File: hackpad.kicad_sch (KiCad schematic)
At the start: 4 parts, among them SW1 SW_Push, SW2 SW_Push, SW3 SW_Push, U1 MOUDLE-SEEEDUINO-XIAO

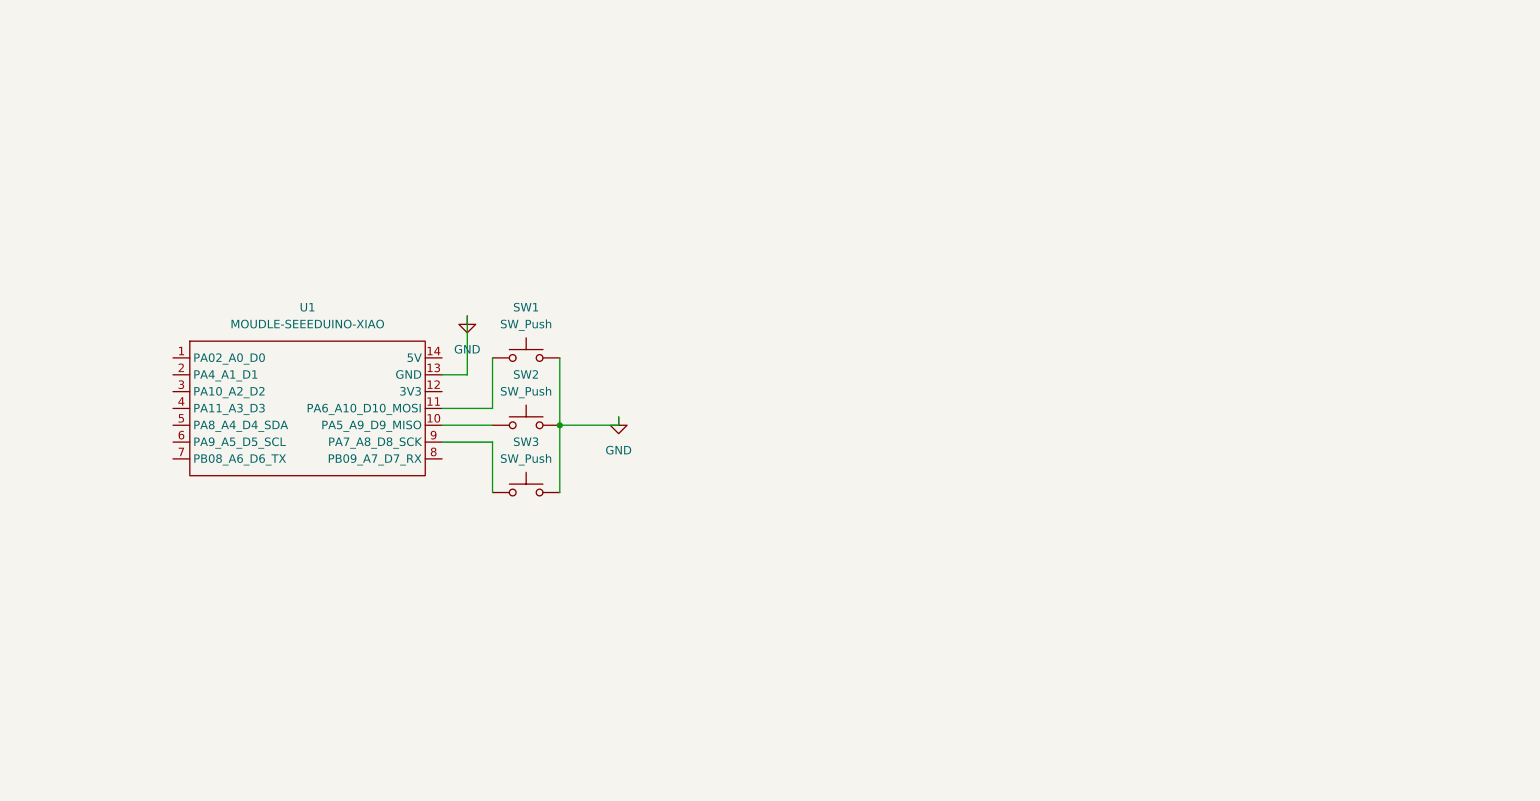
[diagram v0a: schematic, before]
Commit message: made the schematic myself
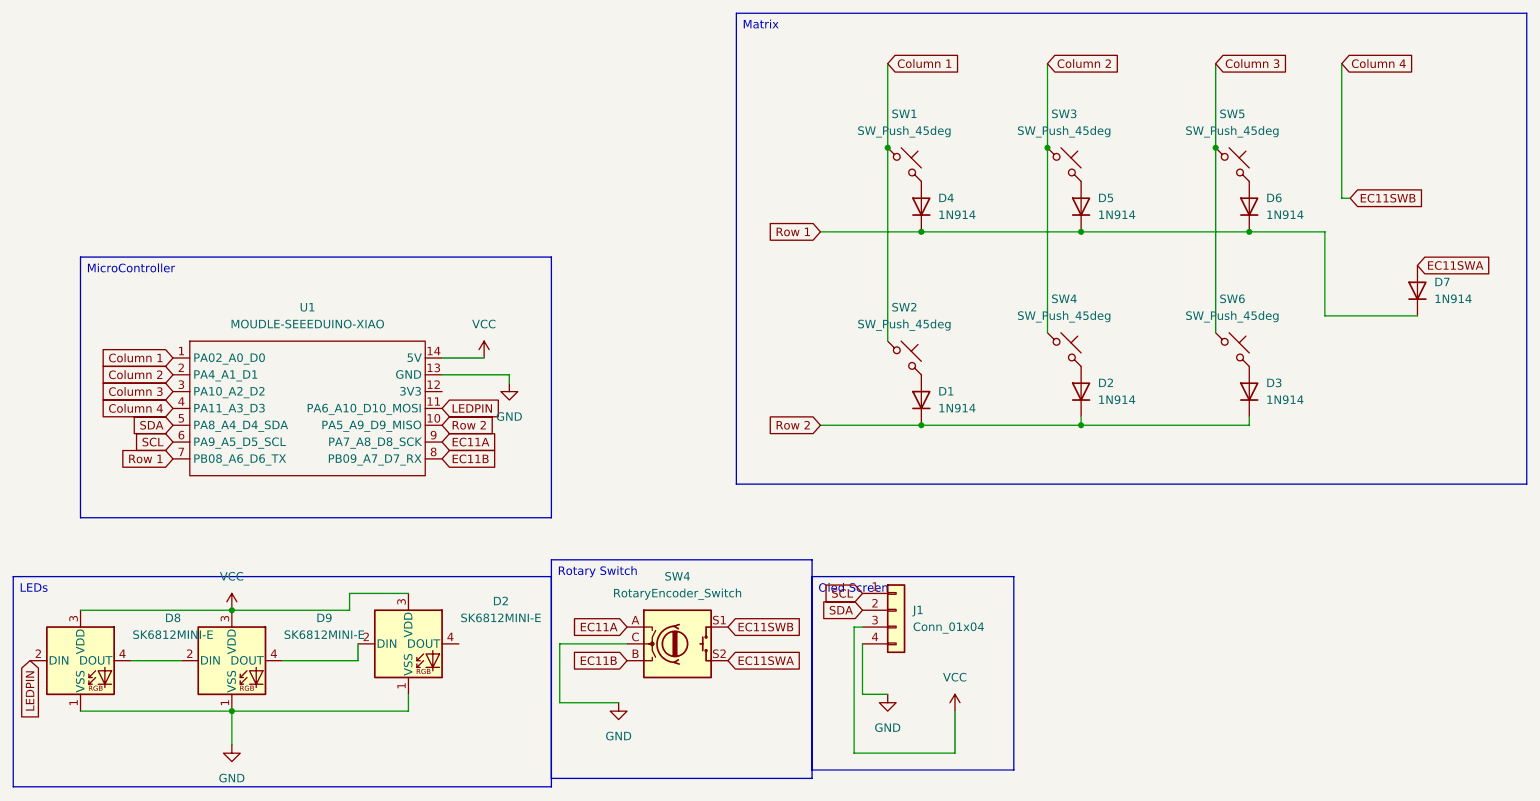
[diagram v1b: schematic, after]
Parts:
- removed SW1, SW2, SW3: SW_Push, Button_Switch_Keyboard:SW_Cherry_MX_1.00u_PCB, symbol Switch:SW_Push
- added D1, D2, D3, D4, D5, D6, D7: 1N914, Diode_THT:D_DO-35_SOD27_P7.62mm_Horizontal, symbol Diode:1N914
- added D2, D8, D9: SK6812MINI-E, LED_SMD:LED_SK6812MINI-E_3.2x2.8mm_P1.5mm_ReverseMount, symbol LED:SK6812MINI-E
- added J1: Conn_01x04, symbol Connector_Generic:Conn_01x04
- added SW1, SW2, SW3, SW4, SW5, SW6: SW_Push_45deg, symbol Switch:SW_Push_45deg
- added SW4: RotaryEncoder_Switch, symbol Device:RotaryEncoder_Switch
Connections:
- net GND: now also D2.1 (VSS), D8.1 (VSS), D9.1 (VSS), J1.4 (Pin_4), SW4.C
- net EC11A: now reaches U1.9 (PA7_A8_D8_SCK)
- net EC11A: now also SW4.A
- net LEDPIN: now reaches U1.11 (PA6_A10_D10_MOSI)
- net LEDPIN: now also D8.2 (DIN)
- net Column 1: now reaches U1.1 (PA02_A0_D0)
- net Column 1: now also SW1.1, SW2.1
- net Row 2: now reaches U1.10 (PA5_A9_D9_MISO)
- net Row 2: now also D1.1 (K), D2.1 (K), D3.1 (K)
- net VCC: now reaches U1.14 (5V)
- net VCC: now also D2.3 (VDD), D8.3 (VDD), D9.3 (VDD), J1.3 (Pin_3)
- net Column 2: now reaches U1.2 (PA4_A1_D1)
- net Column 2: now also SW3.1, SW4.1
- net Column 3: now reaches U1.3 (PA10_A2_D2)
- net Column 3: now also SW5.1, SW6.1
- net Column 4: now reaches U1.4 (PA11_A3_D3)
- net SDA: now reaches U1.5 (PA8_A4_D4_SDA)
- net SDA: now also J1.2 (Pin_2)
- net SCL: now reaches U1.6 (PA9_A5_D5_SCL)
- net SCL: now also J1.1 (Pin_1)
- net Row 1: now reaches U1.7 (PB08_A6_D6_TX)
- net Row 1: now also D4.1 (K), D5.1 (K), D6.1 (K), D7.1 (K)
- net EC11B: now reaches U1.8 (PB09_A7_D7_RX)
- net EC11B: now also SW4.B
- new net: D1.2 (A), SW2.2
- new net: D4.2 (A), SW1.2
- new net: D8.4 (DOUT), D9.2 (DIN)
- new net: D2.2 (DIN), D9.4 (DOUT)
- new net: D6.2 (A), SW5.2
- new net: D3.2 (A), SW6.2
- new net: D5.2 (A), SW3.2
- new net: D2.2 (A), SW4.2
- new net  Column 4: SW4.S1
- new net EC11SWA: D7.2 (A), SW4.S2
